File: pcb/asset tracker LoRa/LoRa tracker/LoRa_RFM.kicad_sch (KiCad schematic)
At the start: 2 parts

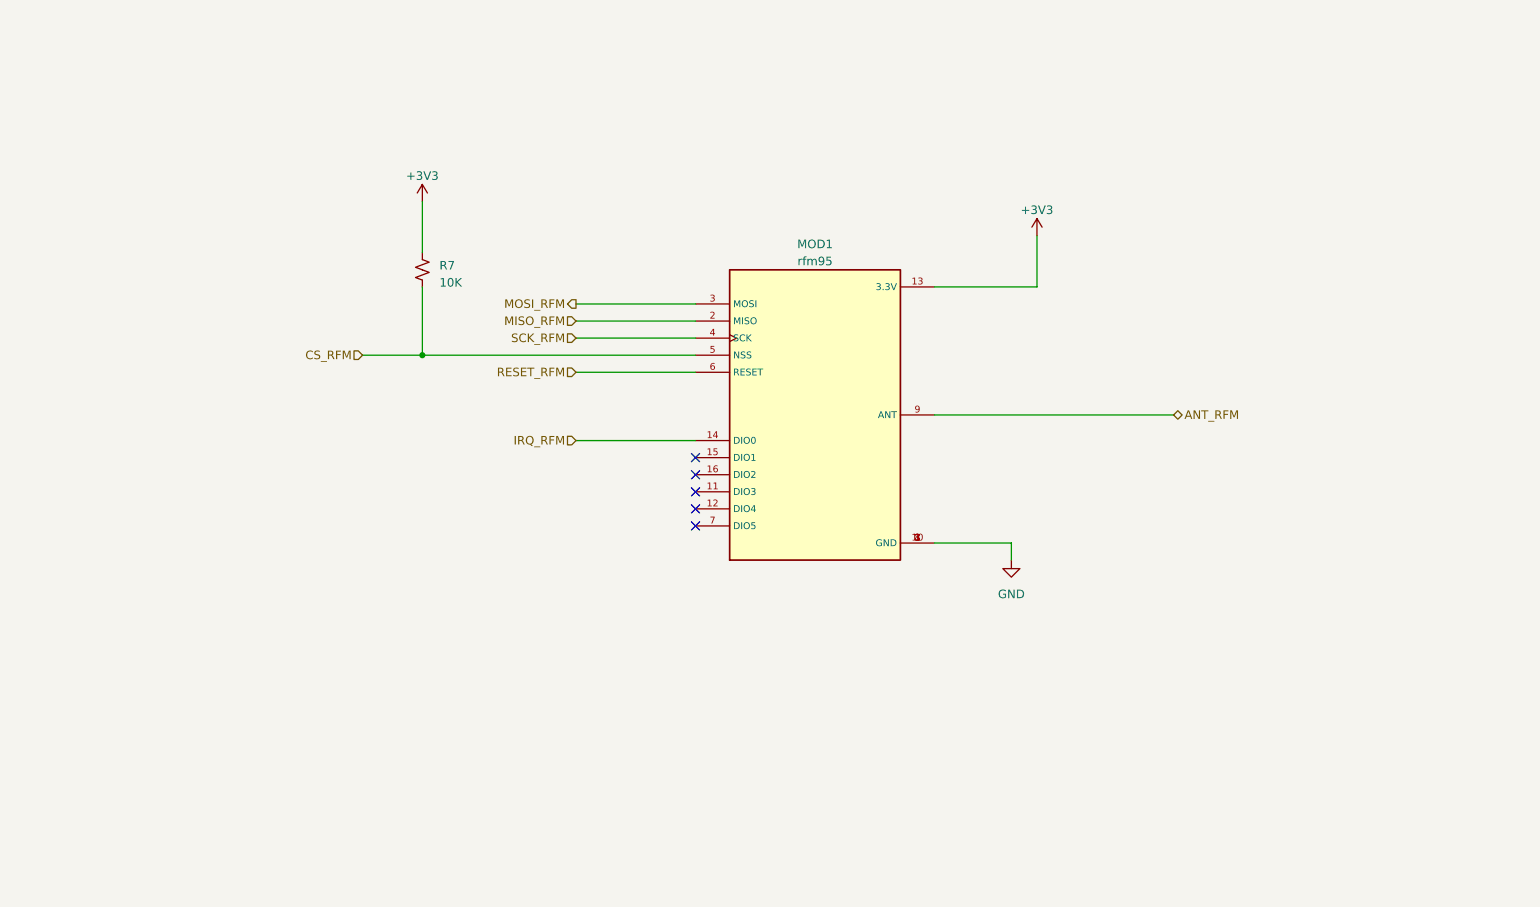
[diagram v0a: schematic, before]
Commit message: pcb kastje
pcb in kastje getekend
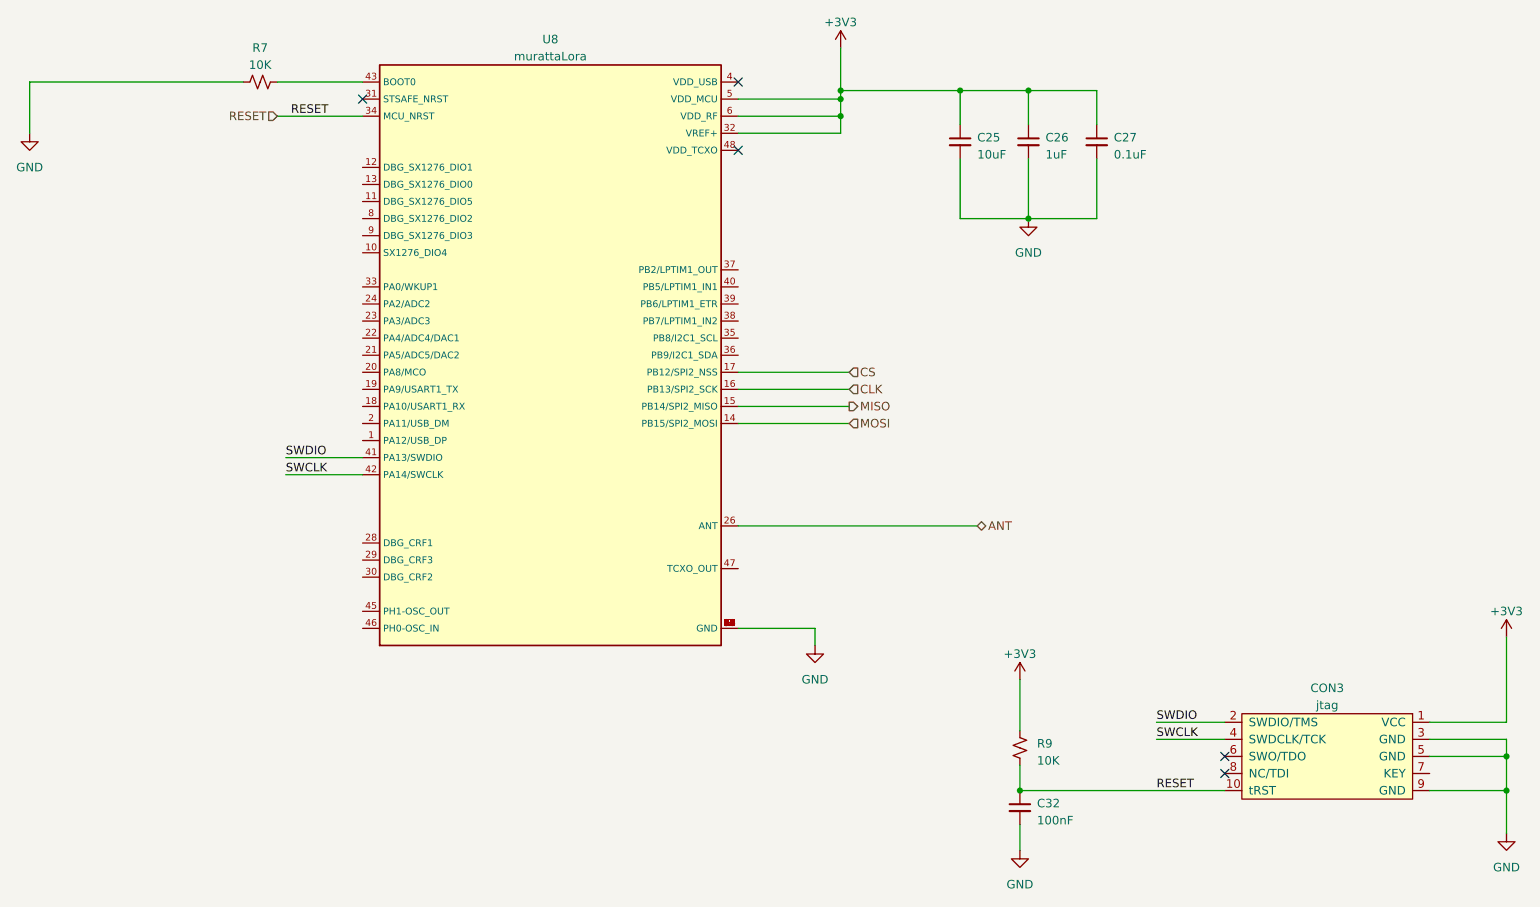
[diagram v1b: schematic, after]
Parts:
- removed MOD1: rfm95, Module:RFM69HW, symbol modulles:rfm95
- added C25: 10uF, vanalles:0603, symbol Device:C_Small
- added C26: 1uF, vanalles:0603, symbol Device:C_Small
- added C27: 0.1uF, vanalles:0603, symbol Device:C_Small
- added C32: 100nF, vanalles:0603, symbol Device:C_Small
- added CON3: jtag, connectors_user:Tag-Connect_TC2050-IDC-FP_2x05_P1.27mm_Vertical, symbol conectors:jtag
- added R9: 10K, vanalles:0603RL, symbol Device:R_Small_US
- added U8: murattaLora, Module:XCVR_CMWX1ZZABZ-078, symbol modulles:murattaLora
- R7: footprint vanalles:0603 -> vanalles:0603RL
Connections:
- net +3V3: now also C25.1, C26.1, C27.1, CON3.1 (VCC), R9.1, U8.32 (VREF+), U8.5 (VDD_MCU), U8.6 (VDD_RF); no longer R7.1
- net GND: now also R7.1, C25.2, C26.2, C27.2, C32.2, CON3.3 (GND), CON3.5 (GND), CON3.9 (GND), U8.25 (GND), U8.27 (GND), U8.3 (GND), U8.44 (GND), U8.49 (GND), U8.50 (GND), U8.51 (GND), U8.52 (GND), U8.53 (GND), U8.54 (GND), U8.55 (GND), U8.56 (GND), U8.57 (GND), U8.7 (GND)
- net CS_RFM: no longer names the net of R7.2
- net CS_RFM: now also U8.43 (BOOT0)
- new net ANT: U8.26 (ANT)
- new net CLK: U8.16 (PB13/SPI2_SCK)
- new net CS: U8.17 (PB12/SPI2_NSS)
- new net MISO: U8.15 (PB14/SPI2_MISO)
- new net MOSI: U8.14 (PB15/SPI2_MOSI)
- new net RESET: C32.1, CON3.10 (tRST), R9.2, U8.34 (MCU_NRST)
- new net SWCLK: CON3.4 (SWDCLK/TCK), U8.42 (PA14/SWCLK)
- new net SWDIO: CON3.2 (SWDIO/TMS), U8.41 (PA13/SWDIO)
